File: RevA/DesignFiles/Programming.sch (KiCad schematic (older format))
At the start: 1 part

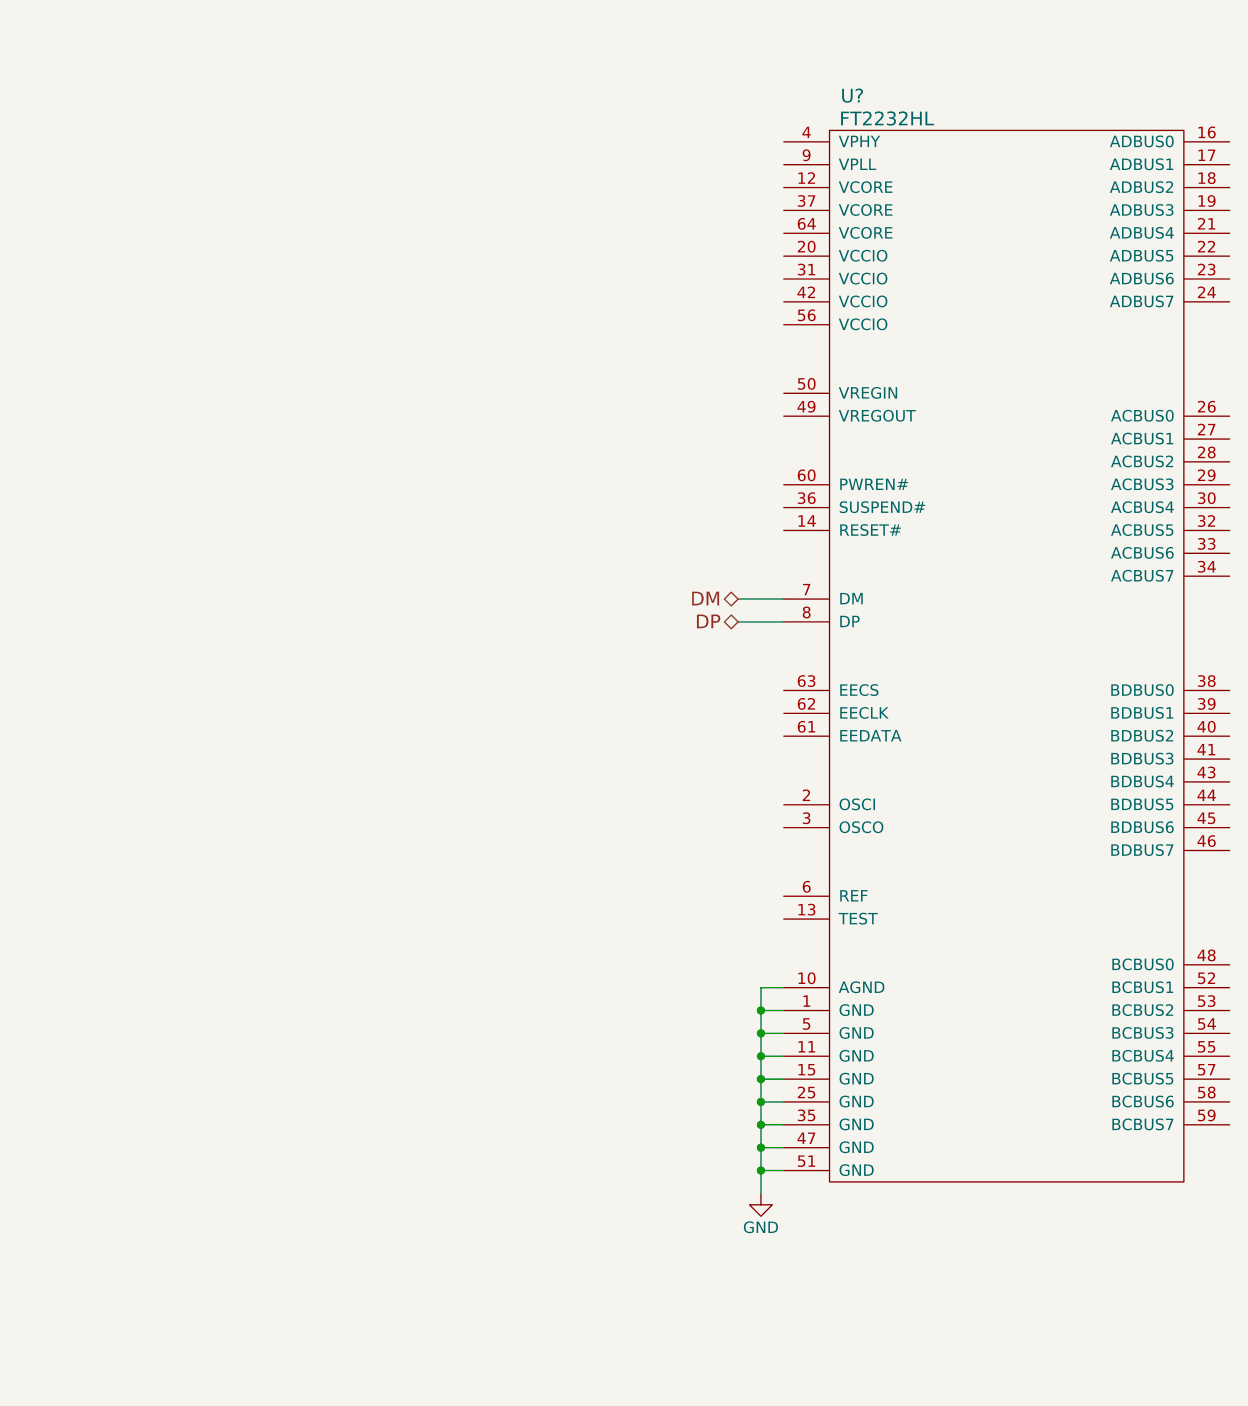
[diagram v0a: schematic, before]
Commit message: more psu stuff for ftdi
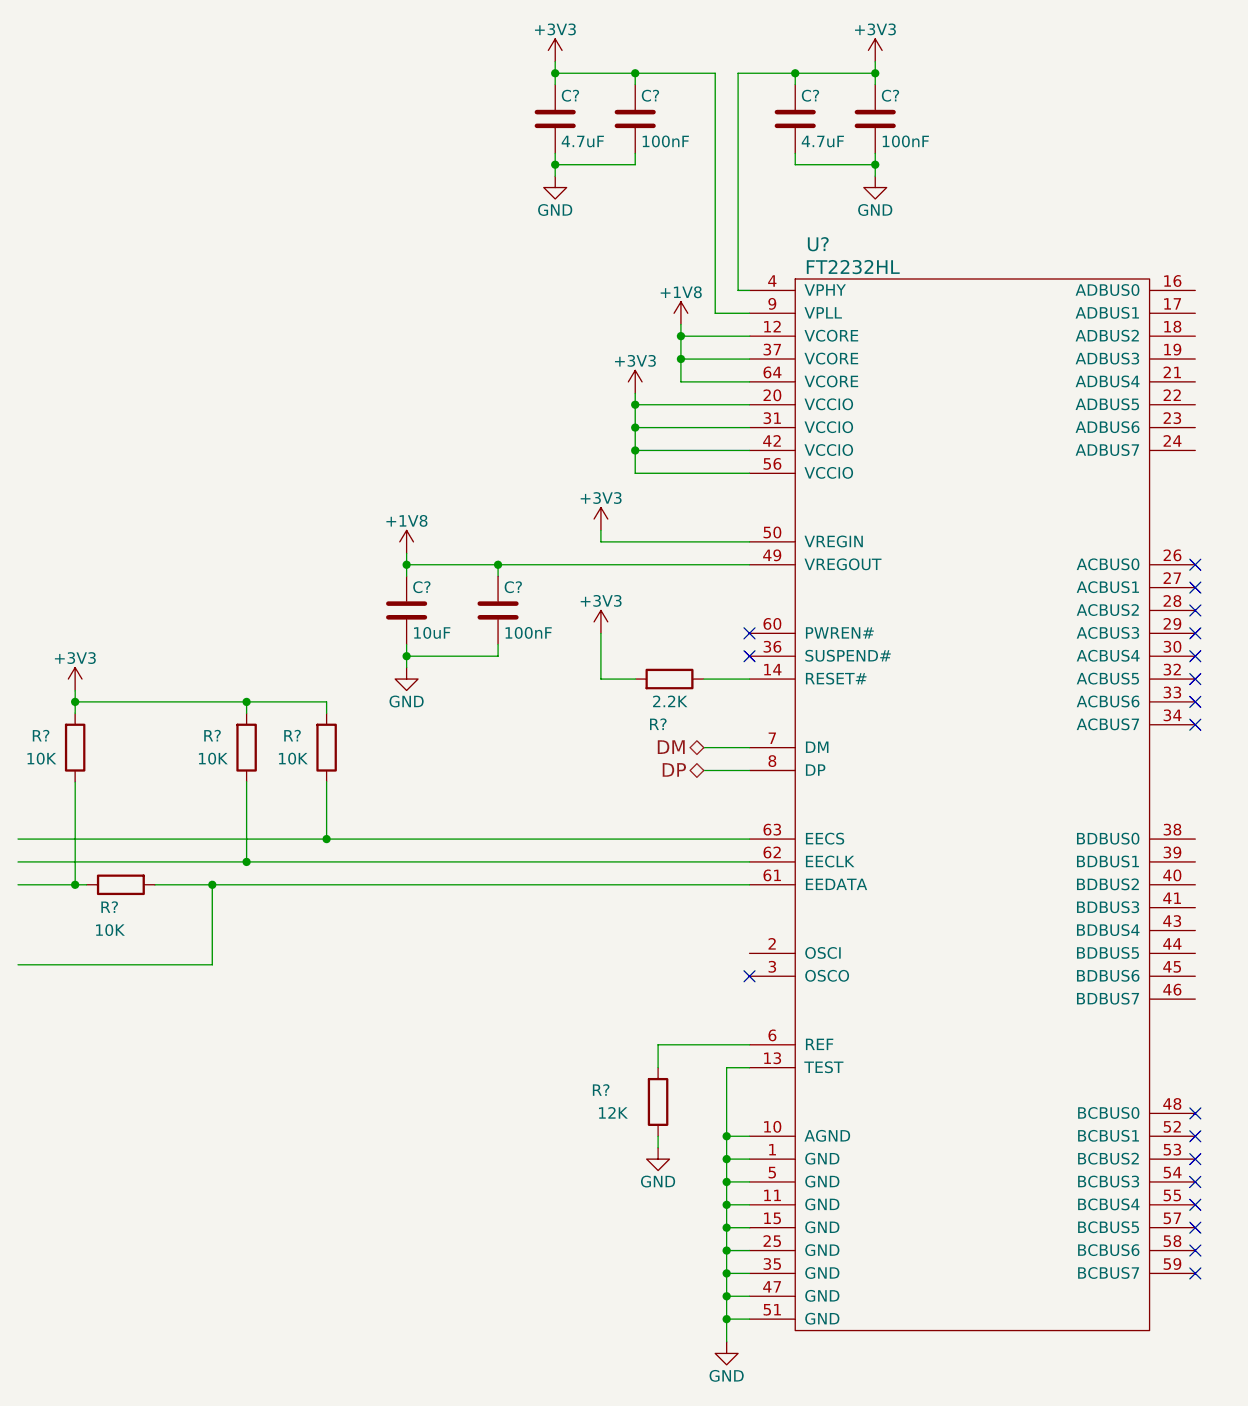
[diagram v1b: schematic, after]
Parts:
- added C? (x3): 100nF, symbol C
- added C?: 10uF, symbol C
- added C? (x2): 4.7uF, symbol C
- added R?: 2.2K, symbol R
- added R?: 12K, symbol R
- added R? (x4): 10K, symbol R
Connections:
- net labels added: +1V8, +3V3
- wire segments 12 -> 65
- no-connect marks 0 -> 19
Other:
- moved on the sheet: U?
